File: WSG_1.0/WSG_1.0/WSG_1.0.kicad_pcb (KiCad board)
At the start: 4 copper layers, 117.5 x 94 mm, 99 parts, among them J1 Conn_01x10, J2 USB_C_Receptacle_USB2.0_16P, J4 Conn_01x02, SW1 SW_Push, SW2 SW_Push, U1 ADS131A04IPBSR, U10 TPS22916CYFPR, U11 W25N04KVZEIR, U12 USBLC6-2SC6, U13 ESP32-S3-MINI-1-N8, U2 DAC60501ZDGSR, U3 INA827AIDGK, U4 INA827AIDGK, U5 INA827AIDGK, U6 TMP235A2DBZR, U7 PQ25180YBGT, U8 TPS63802DLAR, U9 TPS7A2025PDBVR, Y1 SiT8008AI-13-33S-16.384000

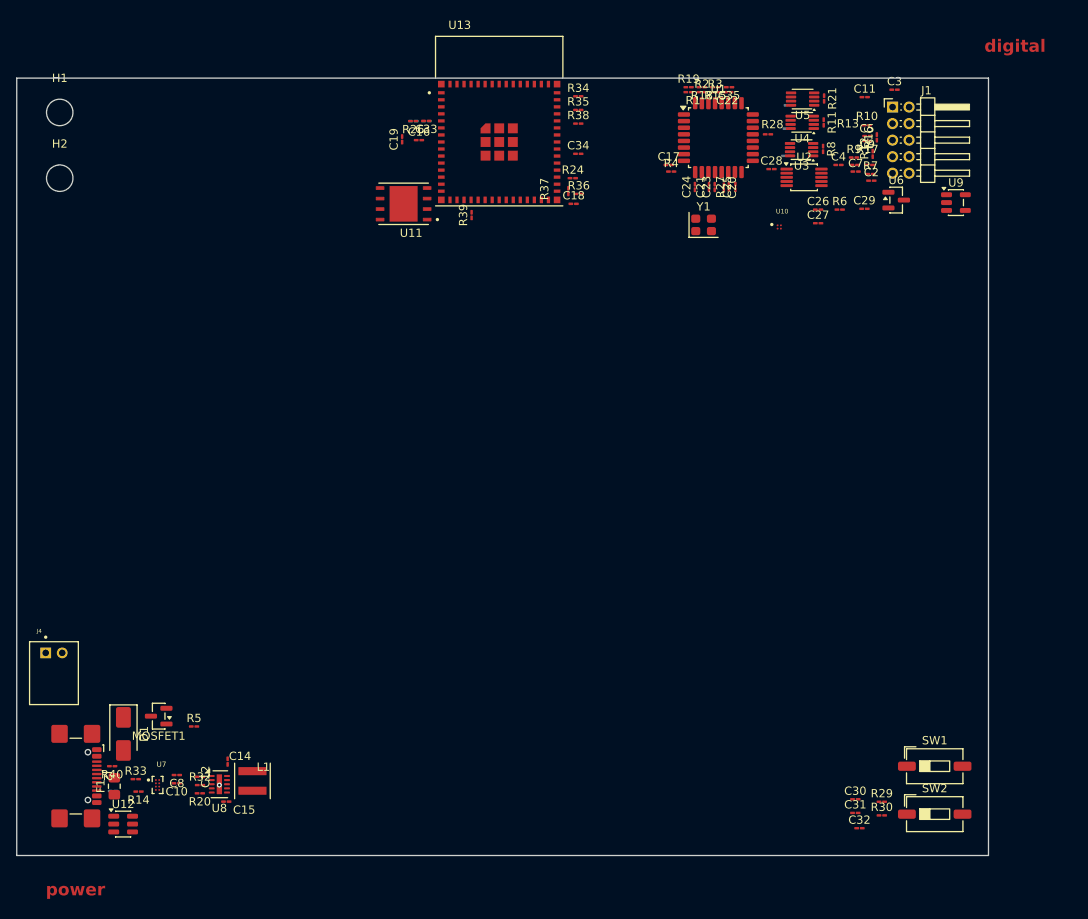
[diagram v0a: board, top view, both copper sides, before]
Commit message: sketch pcb finished
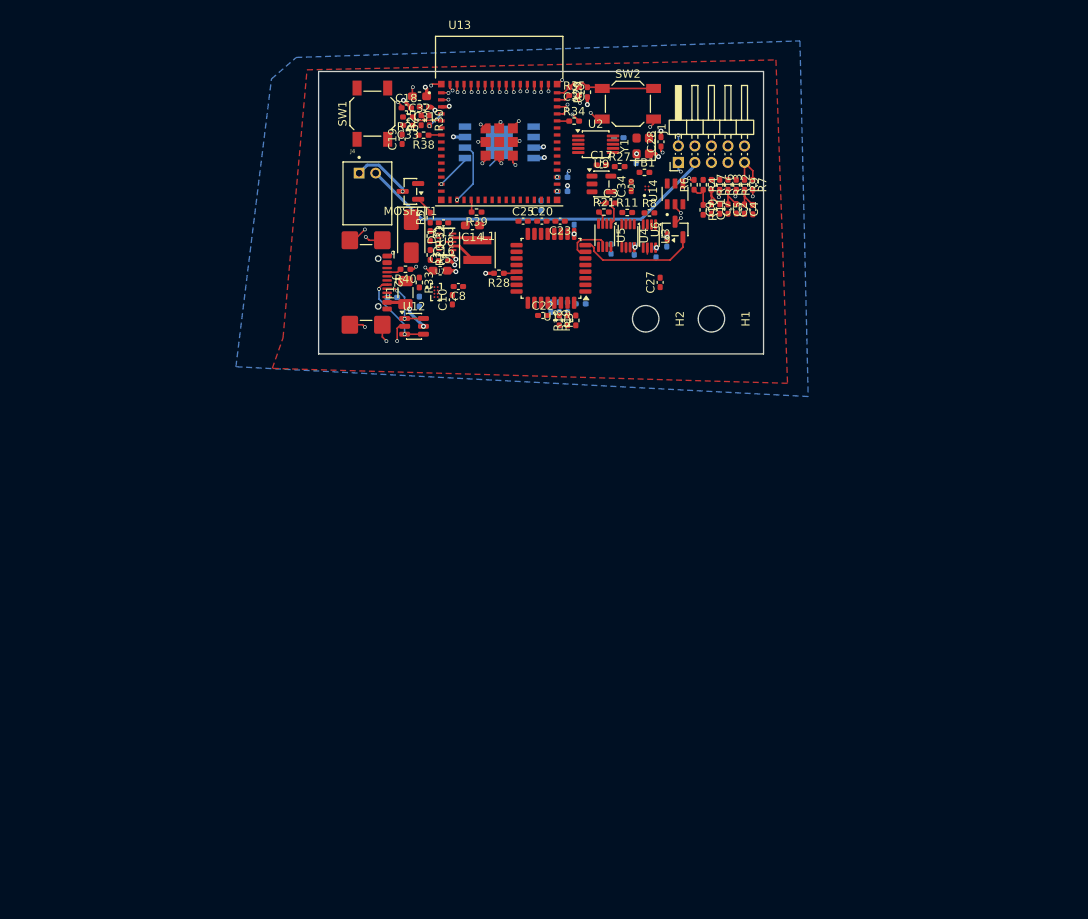
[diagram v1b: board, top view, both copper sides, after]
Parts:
- removed R31: 1M, Resistor_SMD:R_01005_0402Metric_Pad0.57x0.30mm_HandSolder
- added FB1: 0, Resistor_SMD:R_0402_1005Metric_Pad0.72x0.64mm_HandSolder, F.Cu at (127.9, 83.9)
- added U14: TPD4E1U06DBVR, footprints:SOT95P280X145-6N, F.Cu at (131.6, 86.5)
- C1, C10, C11, C12, C13, C16, C17, C18, C19, C2, C20, C22, C23, C25, C27, C28, C3, C30, C31, C33, C34, C4, C5, C6, C7, C8, C9: footprint Capacitor_SMD:C_01005_0402Metric_Pad0.57x0.30mm_HandSolder -> Capacitor_SMD:C_0402_1005Metric_Pad0.74x0.62mm_HandSolder
- C14, C32: value 10uF -> 22uF; footprint Capacitor_SMD:C_01005_0402Metric_Pad0.57x0.30mm_HandSolder -> Capacitor_SMD:C_0603_1608Metric_Pad1.08x0.95mm_HandSolder
- C15: footprint Capacitor_SMD:C_01005_0402Metric_Pad0.57x0.30mm_HandSolder -> Capacitor_SMD:C_0603_1608Metric_Pad1.08x0.95mm_HandSolder
- C21: value 270nF -> 0.1uF; footprint Capacitor_SMD:C_01005_0402Metric_Pad0.57x0.30mm_HandSolder -> Capacitor_SMD:C_0402_1005Metric_Pad0.74x0.62mm_HandSolder; moved to B.Cu
- C24, C26, C29, C35: footprint Capacitor_SMD:C_01005_0402Metric_Pad0.57x0.30mm_HandSolder -> Capacitor_SMD:C_0402_1005Metric_Pad0.74x0.62mm_HandSolder; moved to B.Cu
- F1: value Polyfuse -> 0ZCJ0075AF2E; footprint Fuse:Fuse_0805_2012Metric_Pad1.15x1.40mm_HandSolder -> Fuse:Fuse_1206_3216Metric
- R1, R14, R15, R2, R24, R36, R37: footprint Resistor_SMD:R_01005_0402Metric_Pad0.57x0.30mm_HandSolder -> Resistor_SMD:R_0402_1005Metric_Pad0.72x0.64mm_HandSolder; moved to B.Cu
- R10, R11, R12, R13, R16, R17, R18, R19, R21, R26, R27, R28, R29, R3, R30, R33, R34, R35, R38, R39, R4, R40, R41, R5, R6, R7, R8, R9: footprint Resistor_SMD:R_01005_0402Metric_Pad0.57x0.30mm_HandSolder -> Resistor_SMD:R_0402_1005Metric_Pad0.72x0.64mm_HandSolder
- R20: value 560k -> 511k; footprint Resistor_SMD:R_01005_0402Metric_Pad0.57x0.30mm_HandSolder -> Resistor_SMD:R_0402_1005Metric_Pad0.72x0.64mm_HandSolder
- R25: footprint Resistor_SMD:R_01005_0402Metric_Pad0.57x0.30mm_HandSolder -> Resistor_SMD:R_0402_1005Metric_Pad0.72x0.64mm_HandSolder; moved to F.Cu
- R32: value 100k -> 91k; footprint Resistor_SMD:R_01005_0402Metric_Pad0.57x0.30mm_HandSolder -> Resistor_SMD:R_0402_1005Metric_Pad0.72x0.64mm_HandSolder
- SW1, SW2: footprint Button_Switch_SMD:SW_DIP_SPSTx01_Slide_6.7x4.1mm_W6.73mm_P2.54mm_LowProfile_JPin -> Button_Switch_SMD:SW_SPST_SKQG_WithStem
- U11: footprint footprints:SON127P500X600X80-9N -> footprints:IC_W25N04KVZEIR; moved to B.Cu
- U3, U4, U5: value INA827AIDGK -> INA827AIDGKR
- U7: value PQ25180YBGT -> BQ25180YBGR
- U8: footprint Package_DFN_QFN:DFN-10-1EP_2x3mm_P0.5mm_EP0.64x2.4mm -> footprints:DLA0010A
- moved SW1 104.2 mm to (95.0, 76.8), turned to 90 degrees
- moved C32 103.3 mm to (100.7, 74.7), turned to 180 degrees
- moved R30 100.3 mm to (101.9, 77.6), turned to -90 degrees
- moved C31 100.0 mm to (101.3, 76.0), turned to 180 degrees
- moved SW2 93.6 mm to (125.9, 75.6)
- moved R29 92.9 mm to (121.0, 74.2), turned to 90 degrees
- moved C30 92.6 mm to (119.4, 73.6), turned to 180 degrees
- moved H1 82.7 mm to (136.0, 101.6), turned to -90 degrees
- moved C12 73.2 mm to (103.6, 90.0), turned to 180 degrees
- moved H2 72.9 mm to (128.1, 101.6), turned to -90 degrees
- moved R32 72.0 mm to (102.0, 91.6), turned to -90 degrees
- moved C14 71.3 mm to (107.1, 90.3), turned to 180 degrees
- moved U8 71.1 mm to (103.9, 92.3)
- moved R20 70.8 mm to (102.0, 93.9), turned to -90 degrees
- moved MOSFET1 70.4 mm to (99.6, 86.2)
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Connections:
- C21 pad 1: GND -> 3V3A
- C21 pad 2: VNCP_C -> GND
- C34 pad 2: 3V3 -> Net-(U10-VIN)
- U1 pad 11: VNCP_C -> GND
- U10 pad A2: 3V3 -> Net-(U10-VIN)
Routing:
- net GND: track 0.00 -> 64.6 mm, vias 0 -> 55
- net BATT_N: track 0.00 -> 44.0 mm
- net AIN3P: track 0.00 -> 14.6 mm
- net 3V3: track 0.00 -> 13.3 mm, vias 0 -> 12
- net EN: track 0.00 -> 12.5 mm
- net USB_DM: track 0.00 -> 10.4 mm, vias 0 -> 2
- net FLASH_MISO: track 0.00 -> 7.74 mm, vias 0 -> 1
- net USB_DP: track 0.00 -> 7.44 mm, vias 0 -> 2
- net VREF_1V65: track 0.00 -> 7.24 mm
- net BATT_P: track 0.00 -> 7.16 mm, vias 0 -> 1
- net VBUS: track 0.00 -> 5.89 mm, vias 0 -> 2
- net SIG0: track 0.00 -> 4.62 mm
- net VBAT_SENSE: track 0.00 -> 4.50 mm
- net FLASH_CS: track 0.00 -> 4.34 mm, vias 0 -> 1
- net INP0: track 0.00 -> 4.02 mm
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- added copper zone on In2.Cu, net 3V3
- added copper zone on In2.Cu, net 3V3A
- added copper zone on B.Cu, net GND
- added copper zone on F.Cu, net GND
- added copper zone on In1.Cu, net GND
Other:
- board size 117.5 x 94 mm -> 53.8 x 34.1 mm
- board text removed: "digital"
- board text removed: "power"
